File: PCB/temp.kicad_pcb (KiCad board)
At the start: 2 copper layers, 36 x 40 mm, 41 parts, among them J1 USB_C_Receptacle_USB2.0_14P, J2 MLX90614, J3 OLED, J5 Conn_02x10_Counter_Clockwise, SW1 BOOTSEL, SW2 RST, U1 STM32F103C8Tx, U2 AMS1117-3.3, U3 SRV05-4, Y1 8Mhz, Y3 Crystal

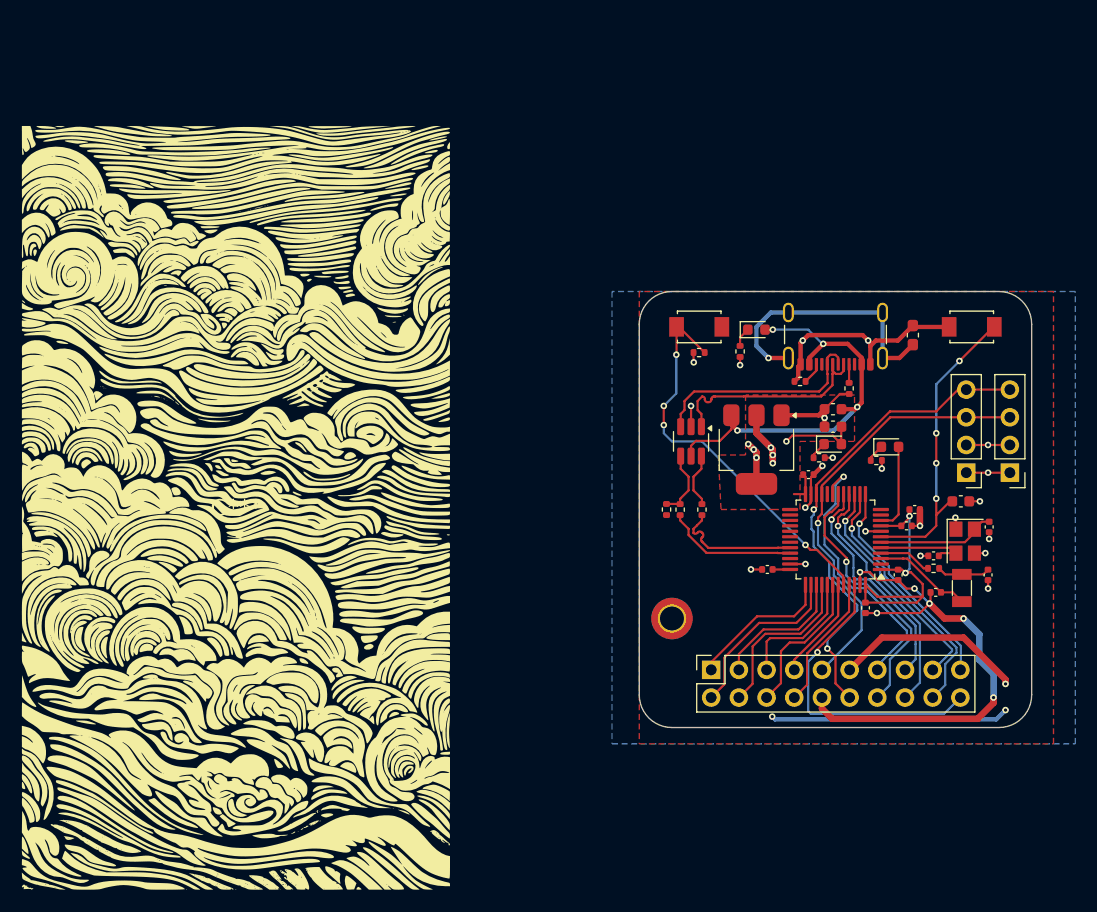
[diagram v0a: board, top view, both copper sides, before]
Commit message: fix
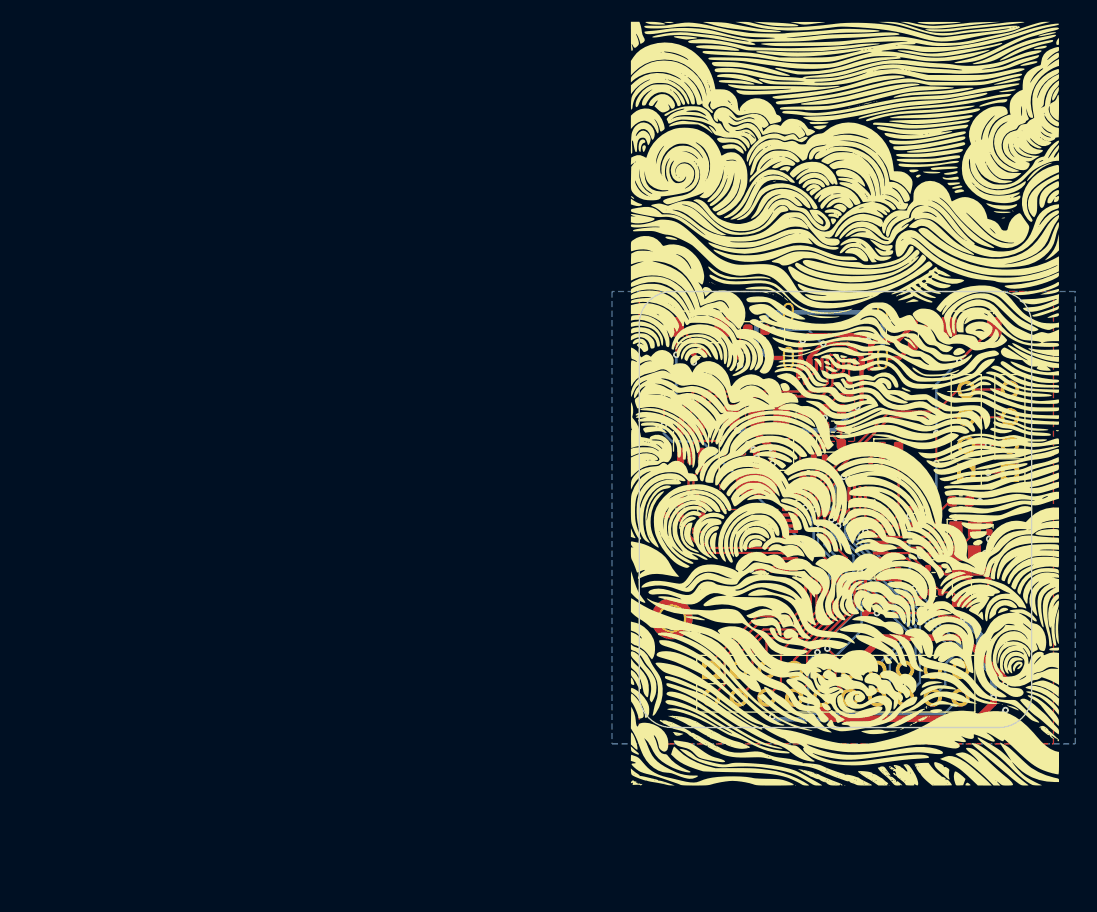
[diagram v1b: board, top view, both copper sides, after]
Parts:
- moved G*** 56.7 mm to (215.9, 110.3)
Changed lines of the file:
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@@
 	(footprint "LOGO"
 		(layer "F.Cu")
-		(at 160 119.846359)
+		(at 215.87 110.29)
 		(property "Reference" "G***"
 			(at 0 0 0)
 			(layer "F.SilkS")
+			(hide yes)
 			(effects
 				(font
